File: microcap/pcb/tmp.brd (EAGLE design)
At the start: 624 parts

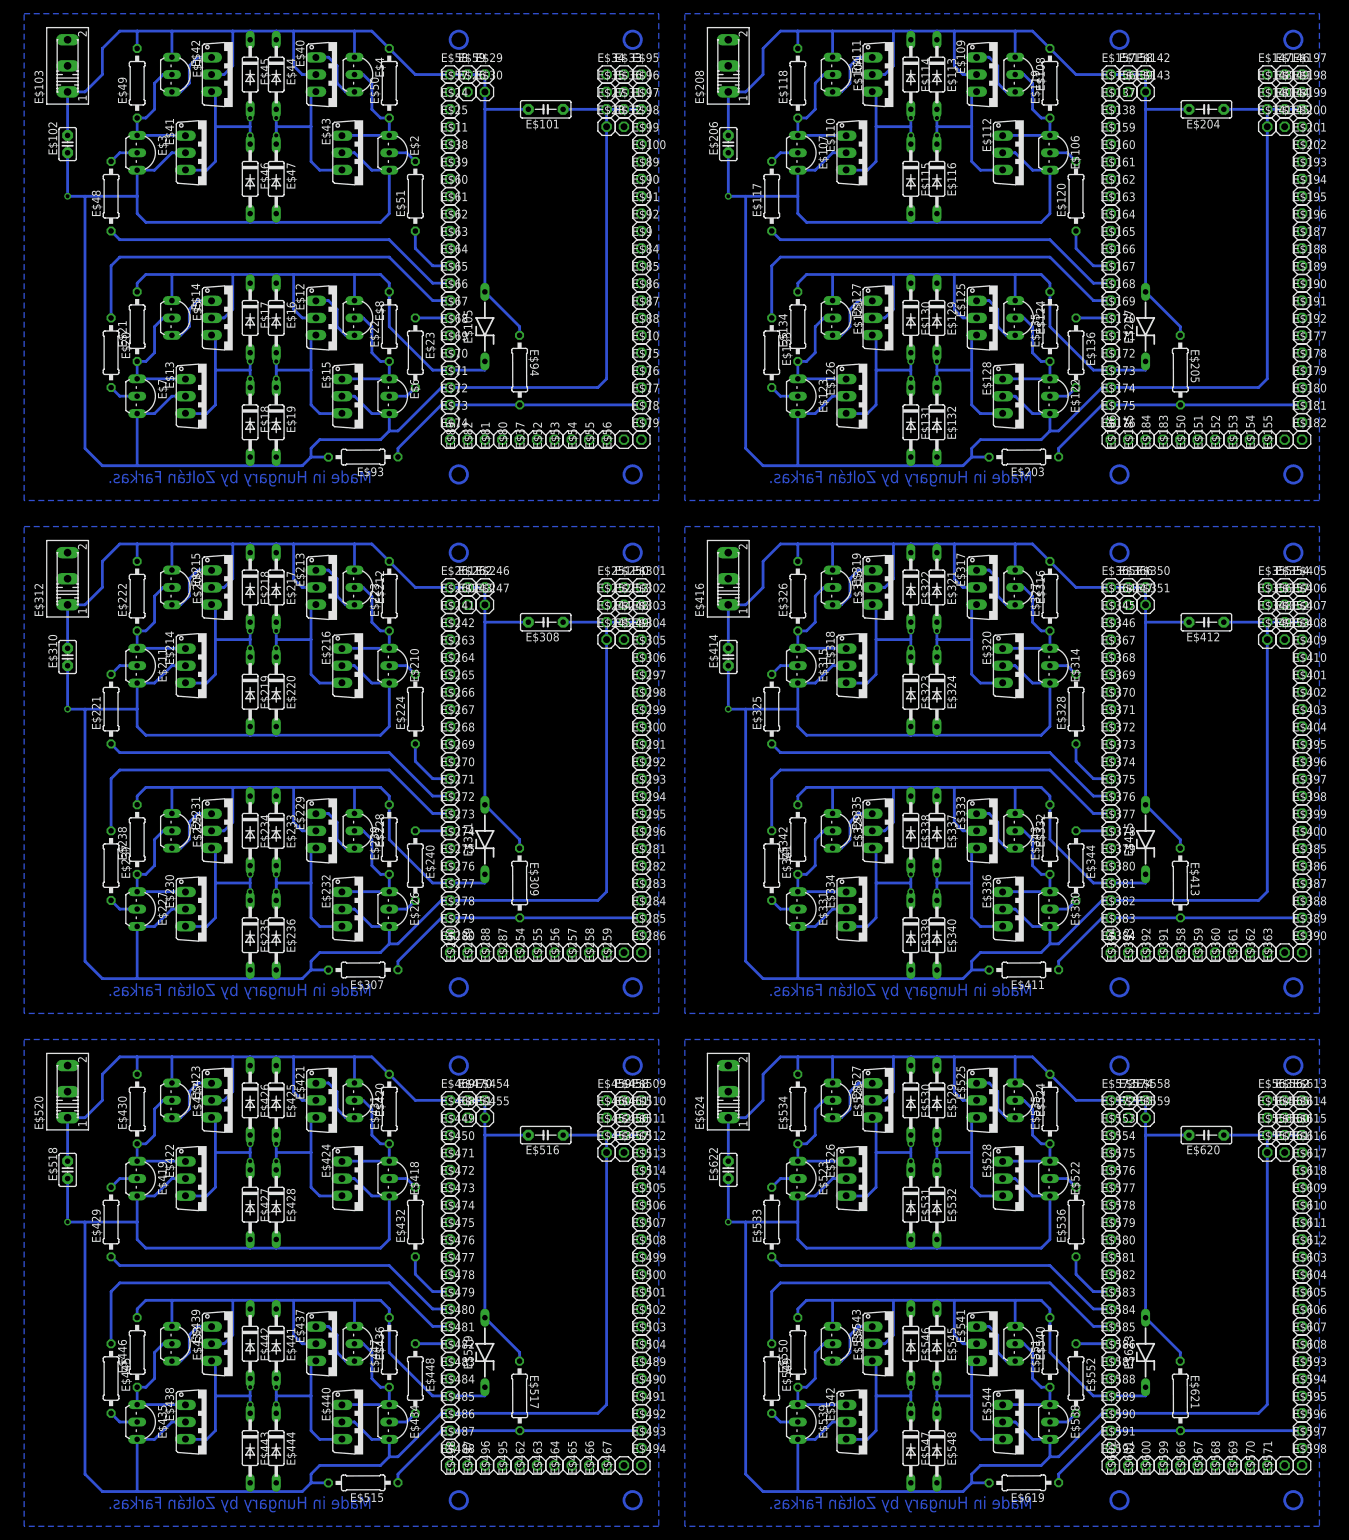
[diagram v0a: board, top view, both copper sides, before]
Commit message: pcb update
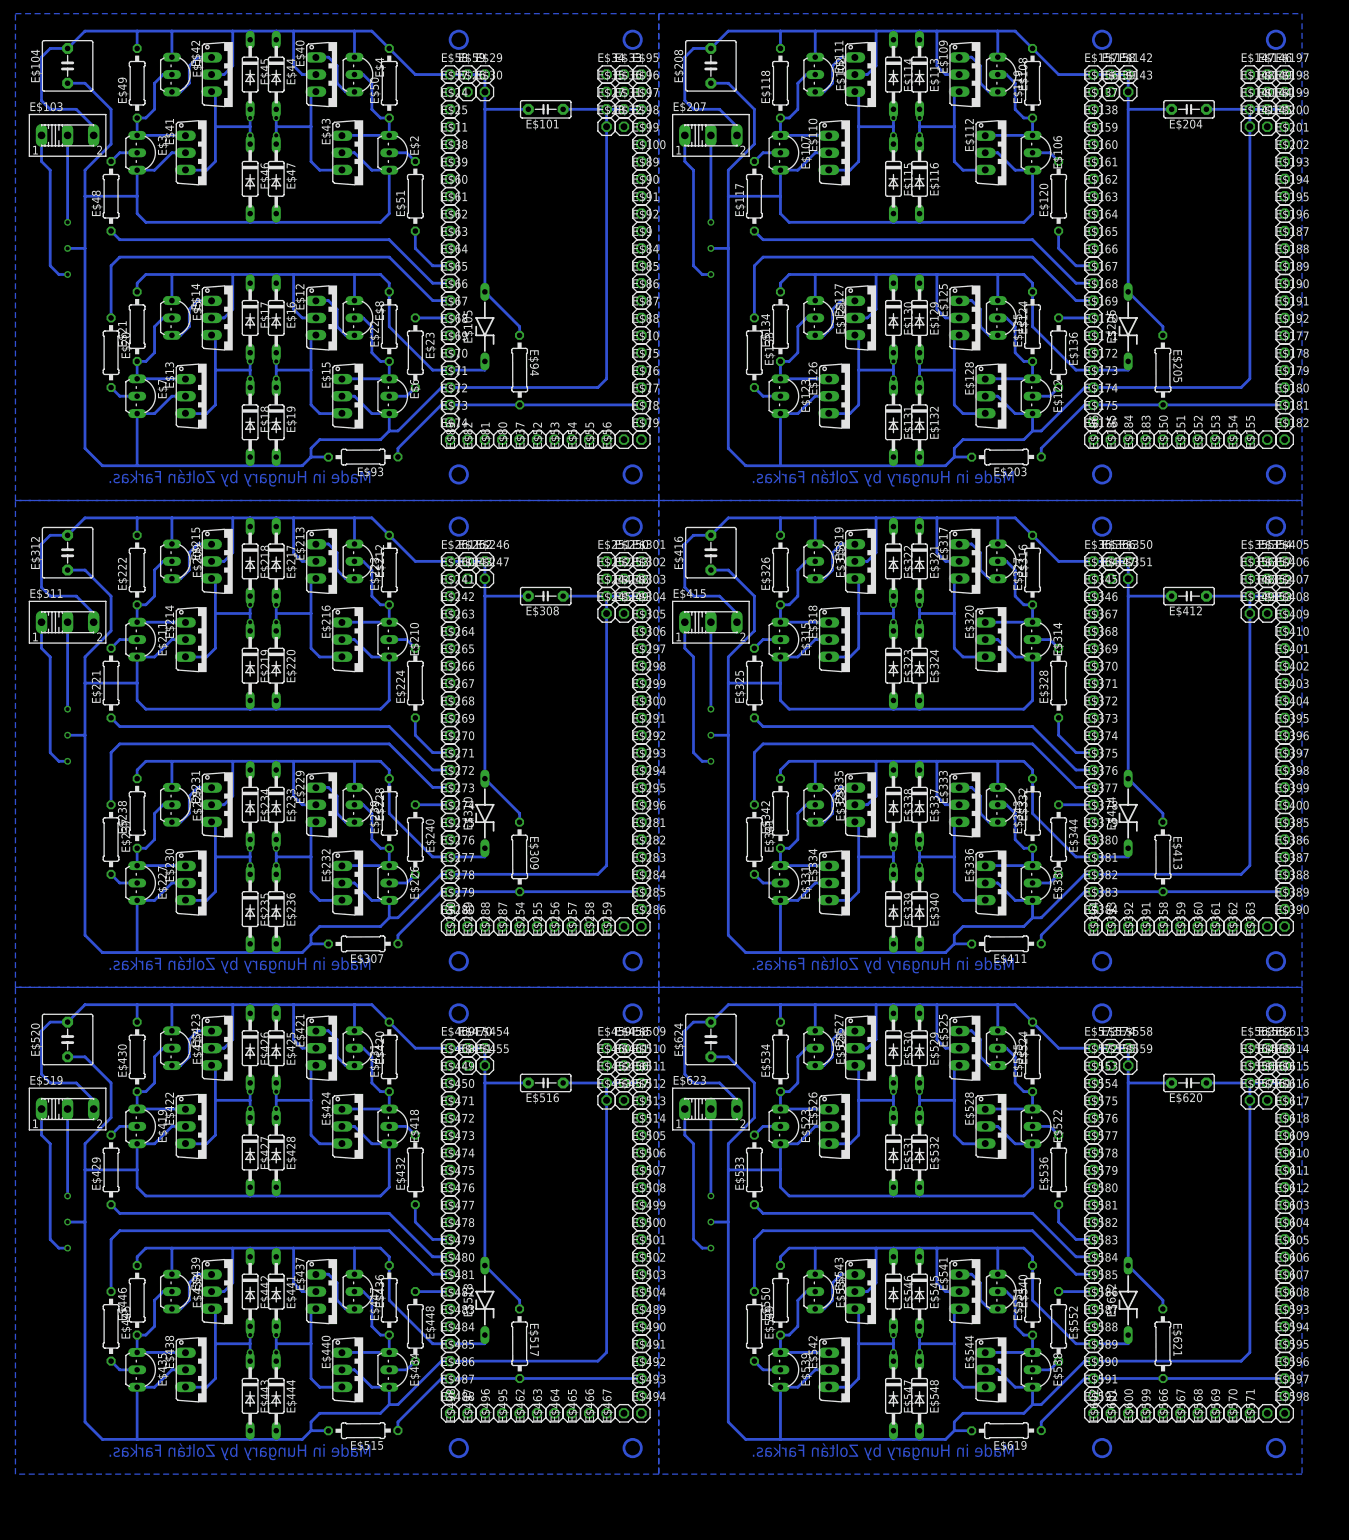
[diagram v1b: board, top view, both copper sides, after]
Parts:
- E$102: device capacitor-wima:C2.5-2 -> transistor:TO92-CBE
- E$104: device transistor:TO92-CBE -> capacitor-wima:C5B7.2
- E$206, E$310, E$414, E$518, E$622: device capacitor-wima:C2.5-2 -> diode:ZDIO-10
- E$207, E$311, E$415, E$519, E$623: device diode:ZDIO-10 -> switch:255SB
- E$208, E$312, E$416, E$520, E$624: device switch:255SB -> capacitor-wima:C5B7.2
- moved E$104 111.8 mm to (27.9, 94.0), turned to 90 degrees
- moved E$102 109.7 mm to (137.2, 92.7), turned to 270 degrees
- moved E$623 72.8 mm to (121.9, -58.4), turned to 0 degrees
- moved E$415 71.0 mm to (121.9, 12.7), turned to 0 degrees
- moved E$519 70.6 mm to (27.9, -58.4), turned to 0 degrees
- moved E$207 69.4 mm to (121.9, 83.8), turned to 0 degrees
- moved E$311 68.7 mm to (27.9, 12.7), turned to 0 degrees
- moved E$310 65.1 mm to (88.9, -15.2)
- moved E$206 64.2 mm to (182.9, 55.9)
- moved E$518 63.9 mm to (88.9, -86.4)
- moved E$414 62.7 mm to (182.9, -15.2)
- moved E$622 61.4 mm to (182.9, -86.4)
- moved E$103 10.2 mm to (27.9, 83.8), turned to 0 degrees
- moved E$525 8.03 mm to (161.3, -49.5)
- moved E$560 8.03 mm to (203.2, -54.6)
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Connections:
- removed net S$100: E$338.A, E$339.C
- removed net S$101: E$337.A, E$340.C
- removed net S$111: E$315.B, E$325.2
- removed net S$125: E$433.B, E$435.C, E$446.1
- removed net S$126: E$433.E
- removed net S$131: E$445.1, E$480.1
- removed net S$132: E$432.1, E$478.1
- removed net S$142: E$434.B, E$448.2
- removed net S$156: E$540.E
- removed net S$157: E$538.C, E$540.B, E$551.1
- removed net S$162: E$533.1, E$583.1
- removed net S$173: E$521.C, E$524.C, E$529.C, E$530.C, E$534.2, E$535.2, E$558.1, E$573.1, E$574.1, E$620.2, E$622.2, E$624.1
- removed net S$32: E$104.E
- removed net S$38: E$121.B, E$123.C, E$134.1
- removed net S$39: E$121.E
- removed net S$49: E$114.A, E$115.C
- removed net S$63: E$212.E
- removed net S$64: E$210.C, E$212.B, E$223.1
- removed net S$69: E$228.E
- removed net S$70: E$226.C, E$228.B, E$239.1
- removed net S$80: E$225.C, E$228.C, E$233.C, E$234.C, E$238.2, E$239.2, E$276.1, E$311.C
- new net S$105: E$330.C, E$332.B, E$343.1
- new net S$117: E$315.B, E$325.2
- new net S$118: E$314.B, E$328.2
- new net S$123: E$313.C, E$316.C, E$321.C, E$322.C, E$326.2, E$327.2, E$350.1, E$365.1, E$366.1, E$412.2, E$415.3, E$416.2
- new net S$124: E$415.1
- new net S$134: E$433.E
- new net S$146: E$433.C, E$436.C, E$441.C, E$442.C, E$446.2, E$447.2, E$484.1, E$518.C
- new net S$147: E$448.1, E$481.1
- new net S$152: E$418.E, E$419.E, E$427.A, E$428.A, E$434.E, E$435.E, E$443.A, E$444.A, E$485.1, E$511.1, E$516.1, E$520.1
- new net S$153: E$519.2
- new net S$175: E$530.A, E$531.C
- new net S$176: E$529.A, E$532.C
- new net S$177: E$537.C, E$540.C, E$545.C, E$546.C, E$550.2, E$551.2, E$588.1, E$622.C
- new net S$178: E$552.1, E$585.1
- new net S$179: E$523.B, E$533.2
- new net S$180: E$522.B, E$536.2
- new net S$181: E$538.B, E$552.2
- new net S$182: E$539.B, E$549.2
- new net S$183: E$522.E, E$523.E, E$531.A, E$532.A, E$538.E, E$539.E, E$547.A, E$548.A, E$589.1, E$615.1, E$620.1, E$624.1
- new net S$184: E$623.2
- new net S$185: E$521.C, E$524.C, E$529.C, E$530.C, E$534.2, E$535.2, E$558.1, E$573.1, E$574.1, E$620.2, E$623.3, E$624.2
- new net S$186: E$623.1
- new net S$29: E$101.1, E$104.1, E$18.A, E$19.A, E$2.E, E$3.E, E$46.A, E$47.A, E$6.E, E$7.E, E$71.1, E$97.1
- new net S$35: E$108.E
- new net S$37: E$106.C, E$108.B, E$119.1
- new net S$47: E$120.1, E$166.1
- new net S$59: E$106.E, E$107.E, E$115.A, E$116.A, E$122.E, E$123.E, E$131.A, E$132.A, E$173.1, E$199.1, E$204.1, E$208.1
- new net S$60: E$207.2
- new net S$65: E$209.B, E$211.C, E$222.1
- new net S$66: E$209.E
- new net S$76: E$233.A, E$236.C
- new net S$88: E$226.B, E$240.2
- new net S$89: E$227.B, E$237.2
- net S$102: now also E$329.B, E$331.C, E$342.1; no longer E$341.1, E$376.1
- net S$103: now also E$329.E; no longer E$328.1, E$374.1
- net S$104: now also E$332.E; no longer E$325.1, E$375.1
- net S$106: now also E$338.A, E$339.C; no longer E$388.1
- net S$107: now also E$337.A, E$340.C; no longer E$322.A, E$323.C
- net S$108: now also E$341.1, E$376.1; no longer E$321.A, E$324.C
- net S$109: now also E$328.1, E$374.1; no longer E$329.C, E$332.C, E$337.C, E$338.C, E$342.2, E$343.2, E$380.1, E$415.C
- net S$110: now also E$325.1, E$375.1; no longer E$344.1, E$377.1
- net S$112: now also E$388.1; no longer E$314.B, E$328.2
- net S$113: now also E$322.A, E$323.C; no longer E$330.B, E$344.2
- net S$114: now also E$321.A, E$324.C; no longer E$331.B, E$341.2
- net S$115: now also E$329.C, E$332.C, E$337.C, E$338.C, E$342.2, E$343.2, E$380.1, E$414.C; no longer E$313.C, E$316.C, E$321.C, E$322.C, E$326.2, E$327.2, E$350.1, E$365.1, E$366.1, E$412.2, E$414.2, E$416.1
- net S$116: now also E$344.1, E$377.1; no longer E$314.E, E$315.E, E$323.A, E$324.A, E$330.E, E$331.E, E$339.A, E$340.A, E$381.1, E$407.1, E$412.1, E$414.1
- net S$119: now also E$330.B, E$344.2; no longer E$417.B, E$419.C, E$430.1
- net S$120: now also E$331.B, E$341.2; no longer E$417.E
- net S$121: now also E$314.E, E$315.E, E$323.A, E$324.A, E$330.E, E$331.E, E$339.A, E$340.A, E$381.1, E$407.1, E$412.1, E$416.1; no longer E$420.E
- net S$122: now also E$415.2; no longer E$418.C, E$420.B, E$431.1
- net S$127: now also E$417.B, E$419.C, E$430.1; no longer E$436.E
- net S$128: now also E$417.E; no longer E$434.C, E$436.B, E$447.1
- net S$129: now also E$420.E; no longer E$442.A, E$443.C
- net S$130: now also E$418.C, E$420.B, E$431.1; no longer E$441.A, E$444.C
- net S$133: now also E$433.B, E$435.C, E$446.1; no longer E$429.1, E$479.1
- net S$135: now also E$436.E; no longer E$492.1
- net S$136: now also E$434.C, E$436.B, E$447.1; no longer E$426.A, E$427.C
- net S$137: now also E$442.A, E$443.C; no longer E$425.A, E$428.C
- net S$138: now also E$441.A, E$444.C; no longer E$433.C, E$436.C, E$441.C, E$442.C, E$446.2, E$447.2, E$484.1, E$519.C
- net S$139: now also E$445.1, E$480.1; no longer E$448.1, E$481.1
- net S$140: now also E$432.1, E$478.1; no longer E$419.B, E$429.2
- net S$141: now also E$429.1, E$479.1; no longer E$418.B, E$432.2
- net S$143: now also E$492.1; no longer E$435.B, E$445.2
- net S$144: now also E$426.A, E$427.C; no longer E$417.C, E$420.C, E$425.C, E$426.C, E$430.2, E$431.2, E$454.1, E$469.1, E$470.1, E$516.2, E$518.2, E$520.1
- net S$145: now also E$425.A, E$428.C; no longer E$418.E, E$419.E, E$427.A, E$428.A, E$434.E, E$435.E, E$443.A, E$444.A, E$485.1, E$511.1, E$516.1, E$518.1
- net S$148: now also E$419.B, E$429.2; no longer E$521.B, E$523.C, E$534.1
- net S$149: now also E$418.B, E$432.2; no longer E$521.E
- net S$150: now also E$434.B, E$448.2; no longer E$524.E
- net S$151: now also E$435.B, E$445.2; no longer E$522.C, E$524.B, E$535.1
- net S$154: now also E$417.C, E$420.C, E$425.C, E$426.C, E$430.2, E$431.2, E$454.1, E$469.1, E$470.1, E$516.2, E$519.3, E$520.2; no longer E$537.B, E$539.C, E$550.1
- net S$155: now also E$519.1; no longer E$537.E
- net S$158: now also E$521.B, E$523.C, E$534.1; no longer E$546.A, E$547.C
- net S$159: now also E$521.E; no longer E$545.A, E$548.C
- net S$160: now also E$524.E; no longer E$549.1, E$584.1
- net S$161: now also E$522.C, E$524.B, E$535.1; no longer E$536.1, E$582.1
- net S$164: now also E$537.B, E$539.C, E$550.1; no longer E$596.1
- net S$165: now also E$537.E; no longer E$530.A, E$531.C
- net S$166: now also E$540.E; no longer E$529.A, E$532.C
- net S$167: now also E$538.C, E$540.B, E$551.1; no longer E$537.C, E$540.C, E$545.C, E$546.C, E$550.2, E$551.2, E$588.1, E$623.C
- net S$168: now also E$546.A, E$547.C; no longer E$552.1, E$585.1
- net S$169: now also E$545.A, E$548.C; no longer E$523.B, E$533.2
- net S$170: now also E$549.1, E$584.1; no longer E$522.B, E$536.2
- net S$171: now also E$536.1, E$582.1; no longer E$538.B, E$552.2
- net S$172: now also E$533.1, E$583.1; no longer E$539.B, E$549.2
- net S$174: now also E$596.1; no longer E$522.E, E$523.E, E$531.A, E$532.A, E$538.E, E$539.E, E$547.A, E$548.A, E$589.1, E$615.1, E$620.1, E$622.1
- net S$20: no longer E$1.C, E$101.2, E$102.2, E$29.1, E$4.C, E$44.C, E$45.C, E$49.2, E$50.2, E$58.1, E$59.1
- net S$25: now also E$1.C, E$101.2, E$103.3, E$104.2, E$29.1, E$4.C, E$44.C, E$45.C, E$49.2, E$50.2, E$58.1, E$59.1; no longer E$101.1, E$102.1, E$18.A, E$19.A, E$2.E, E$3.E, E$46.A, E$47.A, E$6.E, E$7.E, E$71.1, E$97.1
- net S$31: now also E$103.2; no longer E$104.B, E$107.C, E$118.1
- net S$33: now also E$102.B, E$107.C, E$118.1; no longer E$108.E
- net S$34: now also E$102.E; no longer E$106.C, E$108.B, E$119.1
- net S$40: now also E$121.B, E$123.C, E$134.1; no longer E$124.E
- net S$41: now also E$121.E; no longer E$122.C, E$124.B, E$135.1
- net S$42: now also E$124.E; no longer E$130.A, E$131.C
- net S$43: now also E$122.C, E$124.B, E$135.1; no longer E$129.A, E$132.C
- net S$44: now also E$130.A, E$131.C; no longer E$133.1, E$168.1
- net S$45: now also E$129.A, E$132.C; no longer E$120.1, E$166.1
- net S$46: now also E$133.1, E$168.1; no longer E$117.1, E$167.1
- net S$48: now also E$117.1, E$167.1; no longer E$180.1
- net S$50: now also E$180.1; no longer E$113.A, E$116.C
- net S$51: now also E$114.A, E$115.C; no longer E$121.C, E$124.C, E$129.C, E$130.C, E$134.2, E$135.2, E$172.1, E$207.C
- net S$52: now also E$113.A, E$116.C; no longer E$136.1, E$169.1
- net S$53: now also E$121.C, E$124.C, E$129.C, E$130.C, E$134.2, E$135.2, E$172.1, E$206.C; no longer E$107.B, E$117.2
- net S$54: now also E$136.1, E$169.1; no longer E$106.B, E$120.2
- net S$55: now also E$107.B, E$117.2; no longer E$122.B, E$136.2
- net S$56: now also E$106.B, E$120.2; no longer E$123.B, E$133.2
- net S$57: now also E$122.B, E$136.2; no longer E$104.C, E$108.C, E$113.C, E$114.C, E$118.2, E$119.2, E$142.1, E$157.1, E$158.1, E$204.2, E$206.2, E$208.1
- net S$58: now also E$123.B, E$133.2; no longer E$106.E, E$107.E, E$115.A, E$116.A, E$122.E, E$123.E, E$131.A, E$132.A, E$173.1, E$199.1, E$204.1, E$206.1
- net S$61: now also E$102.C, E$108.C, E$113.C, E$114.C, E$118.2, E$119.2, E$142.1, E$157.1, E$158.1, E$204.2, E$207.3, E$208.2; no longer E$209.B, E$211.C, E$222.1
- net S$62: now also E$207.1; no longer E$209.E
- net S$67: now also E$212.E; no longer E$225.B, E$227.C, E$238.1
- net S$68: now also E$210.C, E$212.B, E$223.1; no longer E$225.E
- net S$71: now also E$225.B, E$227.C, E$238.1; no longer E$234.A, E$235.C
- net S$72: now also E$225.E; no longer E$233.A, E$236.C
- net S$73: now also E$228.E; no longer E$237.1, E$272.1
- net S$74: now also E$226.C, E$228.B, E$239.1; no longer E$224.1, E$270.1
- net S$75: now also E$234.A, E$235.C; no longer E$221.1, E$271.1
- net S$77: now also E$237.1, E$272.1; no longer E$284.1
- net S$78: now also E$224.1, E$270.1; no longer E$218.A, E$219.C
- net S$79: now also E$221.1, E$271.1; no longer E$217.A, E$220.C
- net S$81: now also E$284.1; no longer E$240.1, E$273.1
- net S$82: now also E$218.A, E$219.C; no longer E$211.B, E$221.2
- net S$83: now also E$217.A, E$220.C; no longer E$210.B, E$224.2
- net S$84: now also E$225.C, E$228.C, E$233.C, E$234.C, E$238.2, E$239.2, E$276.1, E$310.C; no longer E$226.B, E$240.2
- net S$85: now also E$240.1, E$273.1; no longer E$227.B, E$237.2
- net S$86: now also E$211.B, E$221.2; no longer E$209.C, E$212.C, E$217.C, E$218.C, E$222.2, E$223.2, E$246.1, E$261.1, E$262.1, E$308.2, E$310.2, E$312.1
- net S$87: now also E$210.B, E$224.2; no longer E$210.E, E$211.E, E$219.A, E$220.A, E$226.E, E$227.E, E$235.A, E$236.A, E$277.1, E$303.1, E$308.1, E$310.1
- net S$90: now also E$210.E, E$211.E, E$219.A, E$220.A, E$226.E, E$227.E, E$235.A, E$236.A, E$277.1, E$303.1, E$308.1, E$312.1; no longer E$313.B, E$315.C, E$326.1
- net S$91: now also E$311.2; no longer E$313.E
- net S$92: now also E$209.C, E$212.C, E$217.C, E$218.C, E$222.2, E$223.2, E$246.1, E$261.1, E$262.1, E$308.2, E$311.3, E$312.2; no longer E$316.E
- net S$93: now also E$311.1; no longer E$314.C, E$316.B, E$327.1
- net S$96: now also E$313.B, E$315.C, E$326.1; no longer E$329.B, E$331.C, E$342.1
- net S$97: now also E$313.E; no longer E$329.E
- net S$98: now also E$316.E; no longer E$332.E
- net S$99: now also E$314.C, E$316.B, E$327.1; no longer E$330.C, E$332.B, E$343.1
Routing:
- net S$183: track 0.00 -> 301.2 mm, vias 0 -> 1
- net S$121: track 8.67 -> 301.2 mm, vias 0 -> 1
- net S$90: track 18.8 -> 301.2 mm, vias 0 -> 1
- net S$152: track 19.6 -> 301.2 mm, vias 0 -> 1
- net S$59: track 19.6 -> 301.2 mm, vias 0 -> 1
- net S$29: track 19.6 -> 301.2 mm, vias 0 -> 1
- net S$87: track 285.4 -> 4.34 mm, vias 1 -> 0
- net S$58: track 285.4 -> 4.34 mm, vias 1 -> 0
- net S$145: track 285.4 -> 5.08 mm, vias 1 -> 2
- net S$116: track 285.4 -> 5.08 mm, vias 1 -> 0
- net S$174: track 285.4 -> 39.5 mm, vias 1 -> 0
- net S$185: track 0.00 -> 161.3 mm
- net S$92: track 8.67 -> 161.3 mm
- net S$173: track 151.4 -> 0.00 mm
- net S$57: track 151.4 -> 4.34 mm
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- added copper zone on layer 16, net S$111
- added copper zone on layer 16, net S$142
- added copper zone on layer 16, net S$173
- added copper zone on layer 16, net S$49
- added copper zone on layer 16, net S$80
- removed copper zone on layer 16, net S$105
- removed copper zone on layer 16, net S$134
- removed copper zone on layer 16, net S$163
- removed copper zone on layer 16, net S$47
- removed copper zone on layer 16, net S$76
